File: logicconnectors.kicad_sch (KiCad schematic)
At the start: 28 parts, among them J1 InputConn, J1 USBC Socket, J2 LogicConn2, J3 UART2, J5 HallConn, J6 LogicConn, J7 JTAG, J8 CANConn, U2 USBLC6-2P6, U6 TJA1051T-3

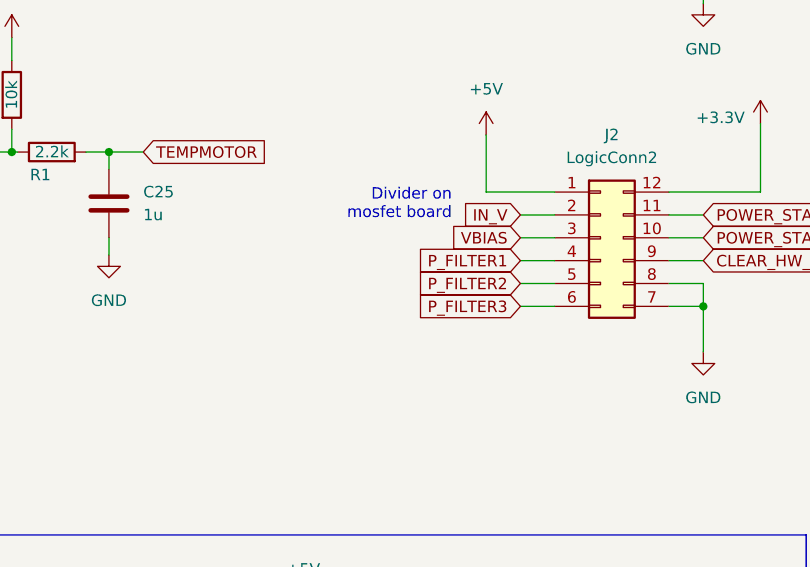
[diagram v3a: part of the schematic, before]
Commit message: initial
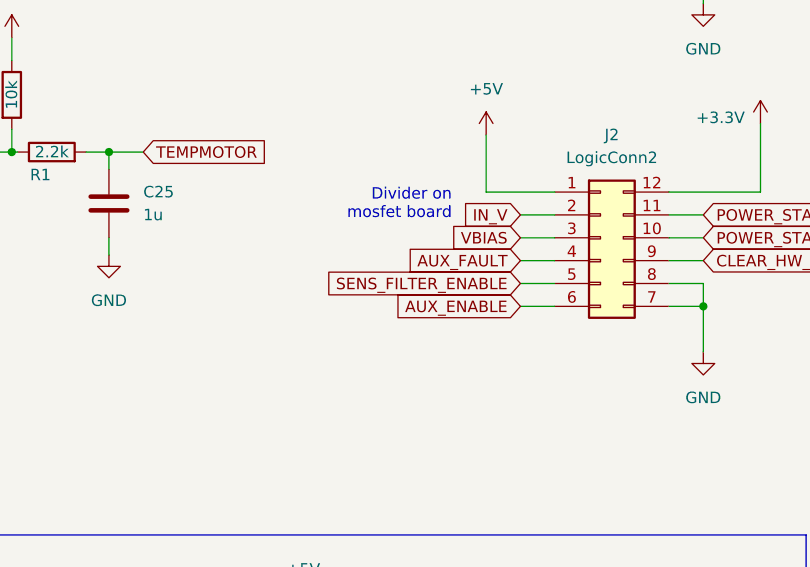
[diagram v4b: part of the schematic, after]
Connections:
- net P_FILTER1 renamed AUX_FAULT
- net P_FILTER2 renamed SENS_FILTER_ENABLE
- net P_FILTER3 renamed AUX_ENABLE
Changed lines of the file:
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@@
+    )
+  )
+  (global_label "SENS_FILTER_ENABLE" (shape input) (at 142.24 101.6 180) (fields_autoplaced)
+    (effects (font (size 1.27 1.27)) (justify right))
+    (property "Intersheetrefs" "${INTERSHEET_REFS}" (at 120.0314 101.6 0)
+      (effects (font (size 1.27 1.27)) (justify right) hide)
     )
   )
@@
     )
   )
+  (global_label "AUX_FAULT" (shape input) (at 142.24 99.06 180) (fields_autoplaced)
+    (effects (font (size 1.27 1.27)) (justify right))
+    (property "Intersheetrefs" "${INTERSHEET_REFS}" (at 129.8888 99.06 0)
+      (effects (font (size 1.27 1.27)) (justify right) hide)
+    )
+  )
   (global_label "MOSTEMP1" (shape input) (at 163.83 52.705 0) (fields_autoplaced)
     (effects (font (size 1.27 1.27)) (justify left))
@@
     )
   )
-  (global_label "P_FILTER3" (shape input) (at 142.24 104.14 180) (fields_autoplaced)
-    (effects (font (size 1.27 1.27)) (justify right))
-    (property "Intersheetrefs" "${INTERSHEET_REFS}" (at 130.4332 104.14 0)
-      (effects (font (size 1.27 1.27)) (justify right) hide)
-    )
-  )
   (global_label "CANTx" (shape input) (at 101.6 160.02 180) (fields_autoplaced)
     (effects (font (size 1.27 1.27)) (justify right))
@@
     )
   )
-  (global_label "P_FILTER1" (shape input) (at 142.24 99.06 180) (fields_autoplaced)
-    (effects (font (size 1.27 1.27)) (justify right))
-    (property "Intersheetrefs" "${INTERSHEET_REFS}" (at 130.4332 99.06 0)
-      (effects (font (size 1.27 1.27)) (justify right) hide)
-    )
-  )
   (global_label "TX_SCL_MOSI" (shape input) (at 38.1 52.07 0) (fields_autoplaced)
     (effects (font (size 1.27 1.27)) (justify left))
@@
     )
   )
-  (global_label "P_FILTER2" (shape input) (at 142.24 101.6 180) (fields_autoplaced)
-    (effects (font (size 1.27 1.27)) (justify right))
-    (property "Intersheetrefs" "${INTERSHEET_REFS}" (at 130.4332 101.6 0)
-      (effects (font (size 1.27 1.27)) (justify right) hide)
-    )
-  )
   (global_label "TX_EXT2" (shape input) (at 41.91 92.075 0) (fields_autoplaced)
     (effects (font (size 1.27 1.27)) (justify left))
@@
     )
   )
+  (global_label "AUX_ENABLE" (shape input) (at 142.24 104.14 180) (fields_autoplaced)
+    (effects (font (size 1.27 1.27)) (justify right))
+    (property "Intersheetrefs" "${INTERSHEET_REFS}" (at 128.377 104.14 0)
+      (effects (font (size 1.27 1.27)) (justify right) hide)
+    )
+  )

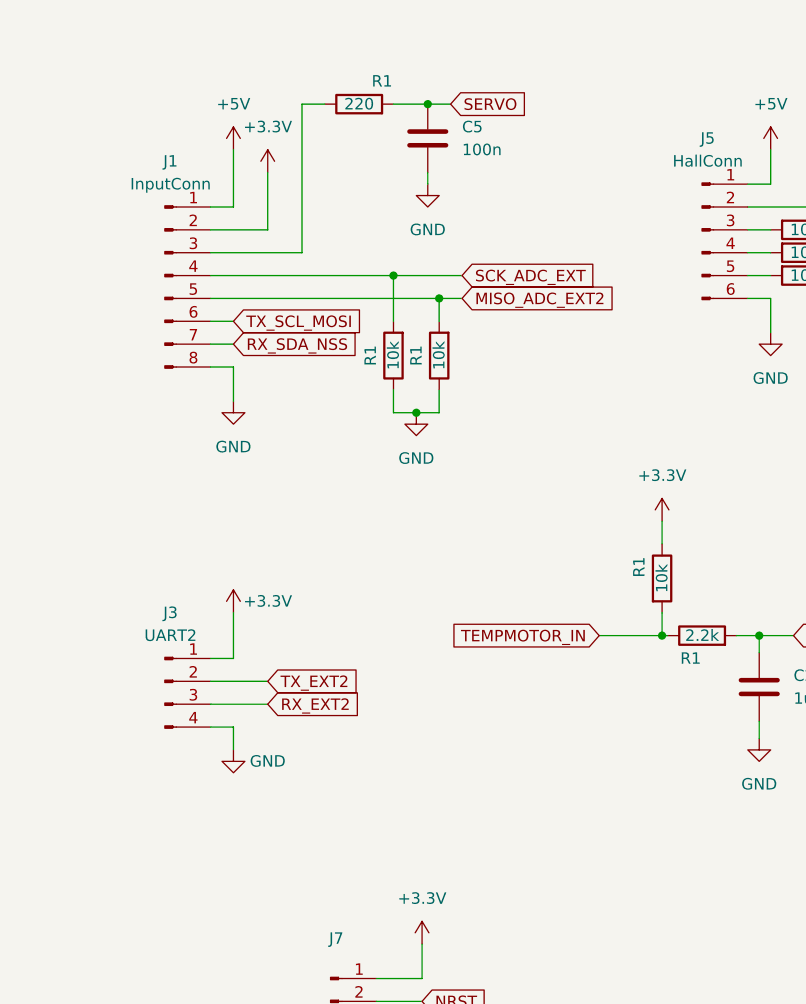
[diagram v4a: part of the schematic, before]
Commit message: jlcpcb
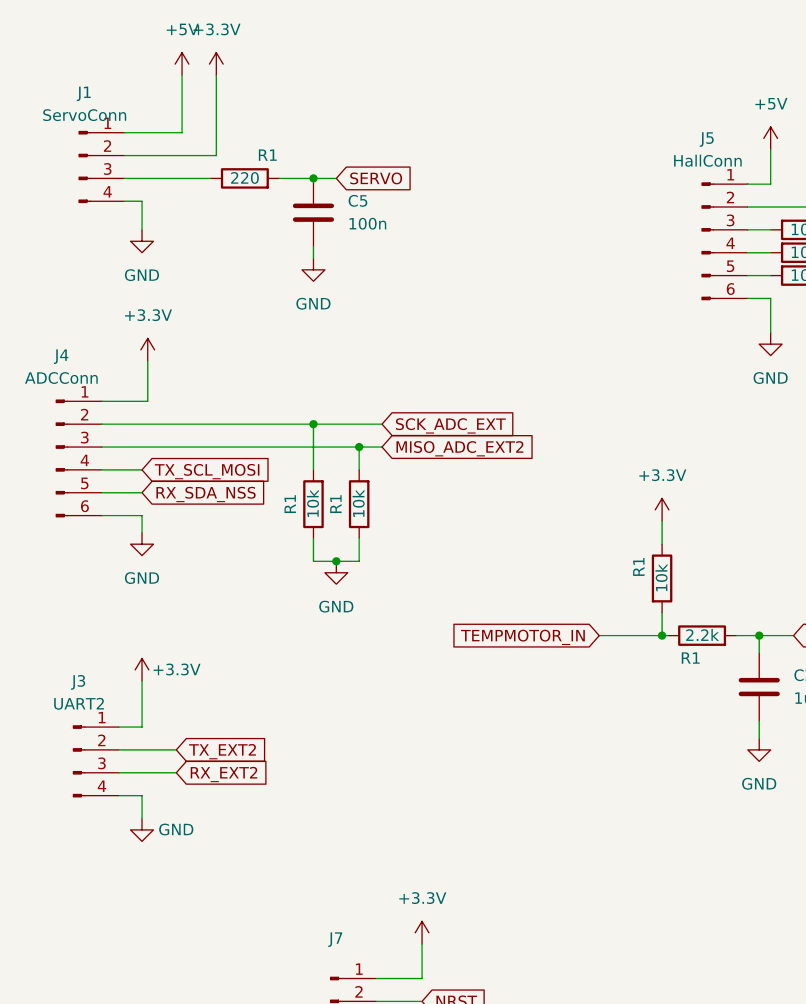
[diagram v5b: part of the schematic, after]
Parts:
- removed J1: InputConn, Connector_PinHeader_2.54mm:PinHeader_1x08_P2.54mm_Horizontal, symbol Connector:Conn_01x08_Pin
- added J1: ServoConn, Connector_JST:JST_EH_S4B-EH_1x04_P2.50mm_Horizontal, symbol Connector:Conn_01x04_Pin
- added J4: ADCConn, Connector_JST:JST_EH_S6B-EH_1x06_P2.50mm_Horizontal, symbol Connector:Conn_01x06_Pin
- C27: MPN (none) -> C377773
- J1: MPN (none) -> C2765186
- J2: MPN (none) -> C225521
- J3, J8: footprint Connector_PinHeader_2.54mm:PinHeader_1x04_P2.54mm_Horizontal -> Connector_JST:JST_EH_S4B-EH_1x04_P2.50mm_Horizontal; MPN (none) -> C265068
- J5: footprint Connector_PinHeader_2.54mm:PinHeader_1x06_P2.54mm_Horizontal -> Connector_JST:JST_EH_S6B-EH_1x06_P2.50mm_Horizontal; MPN (none) -> C495208
- J6: MPN (none) -> C2685199
- J7: MPN (none) -> C124379
- R1: MPN (none) -> C17557
- R1: MPN (none) -> C17408
- R4: MPN (none) -> C17561
- R5: MPN (none) -> C118848
- U2: MPN (none) -> C2827693
- U6: footprint Package_SO:SOIC-8_3.9x4.9mm_P1.27mm -> Package_SO:SOP-8_3.9x4.9mm_P1.27mm; MPN (none) -> C5342108
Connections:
- net +3.3V: now also J1.2 (Pin_2), J4.1 (Pin_1)
- net +5V: now also J1.1 (Pin_1)
- net GND: now also J1.4 (Pin_4), J4.6 (Pin_6)
- net MISO_ADC_EXT2: now also J4.3 (Pin_3)
- net RX_SDA_NSS: now also J4.5 (Pin_5)
- net SCK_ADC_EXT: now also J4.2 (Pin_2)
- net TX_SCL_MOSI: now also J4.4 (Pin_4)
- net at R1.1: now also J1.3 (Pin_3)
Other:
- moved on the sheet: C5, J3, R1

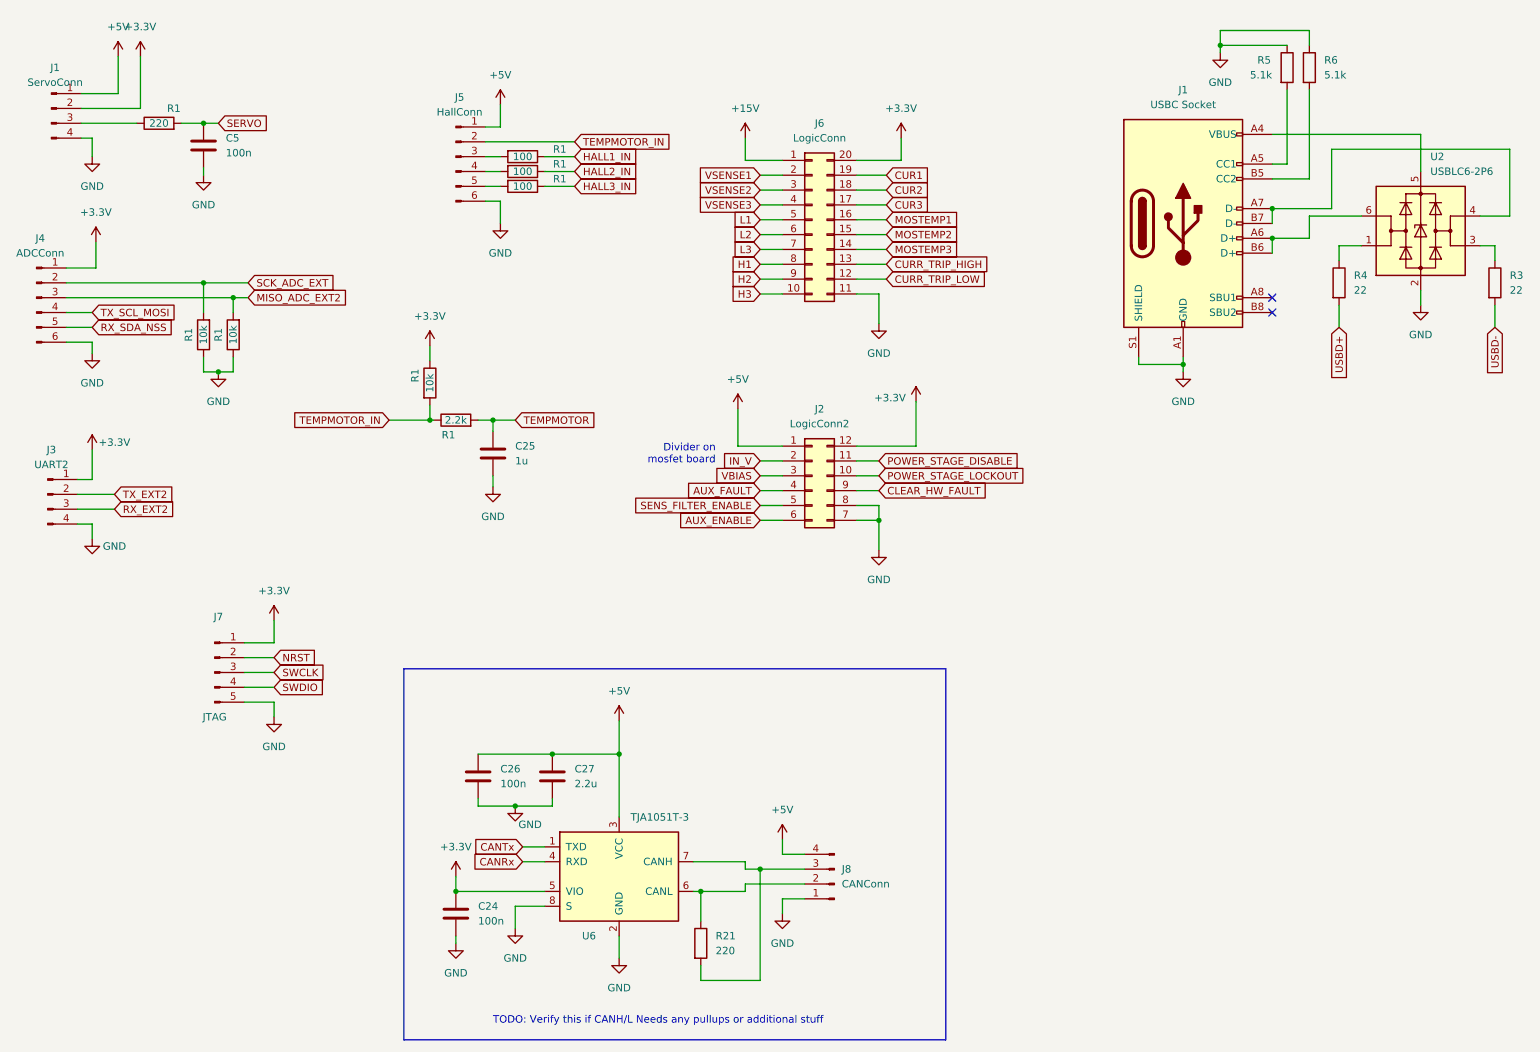
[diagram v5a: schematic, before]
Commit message: routinglogic
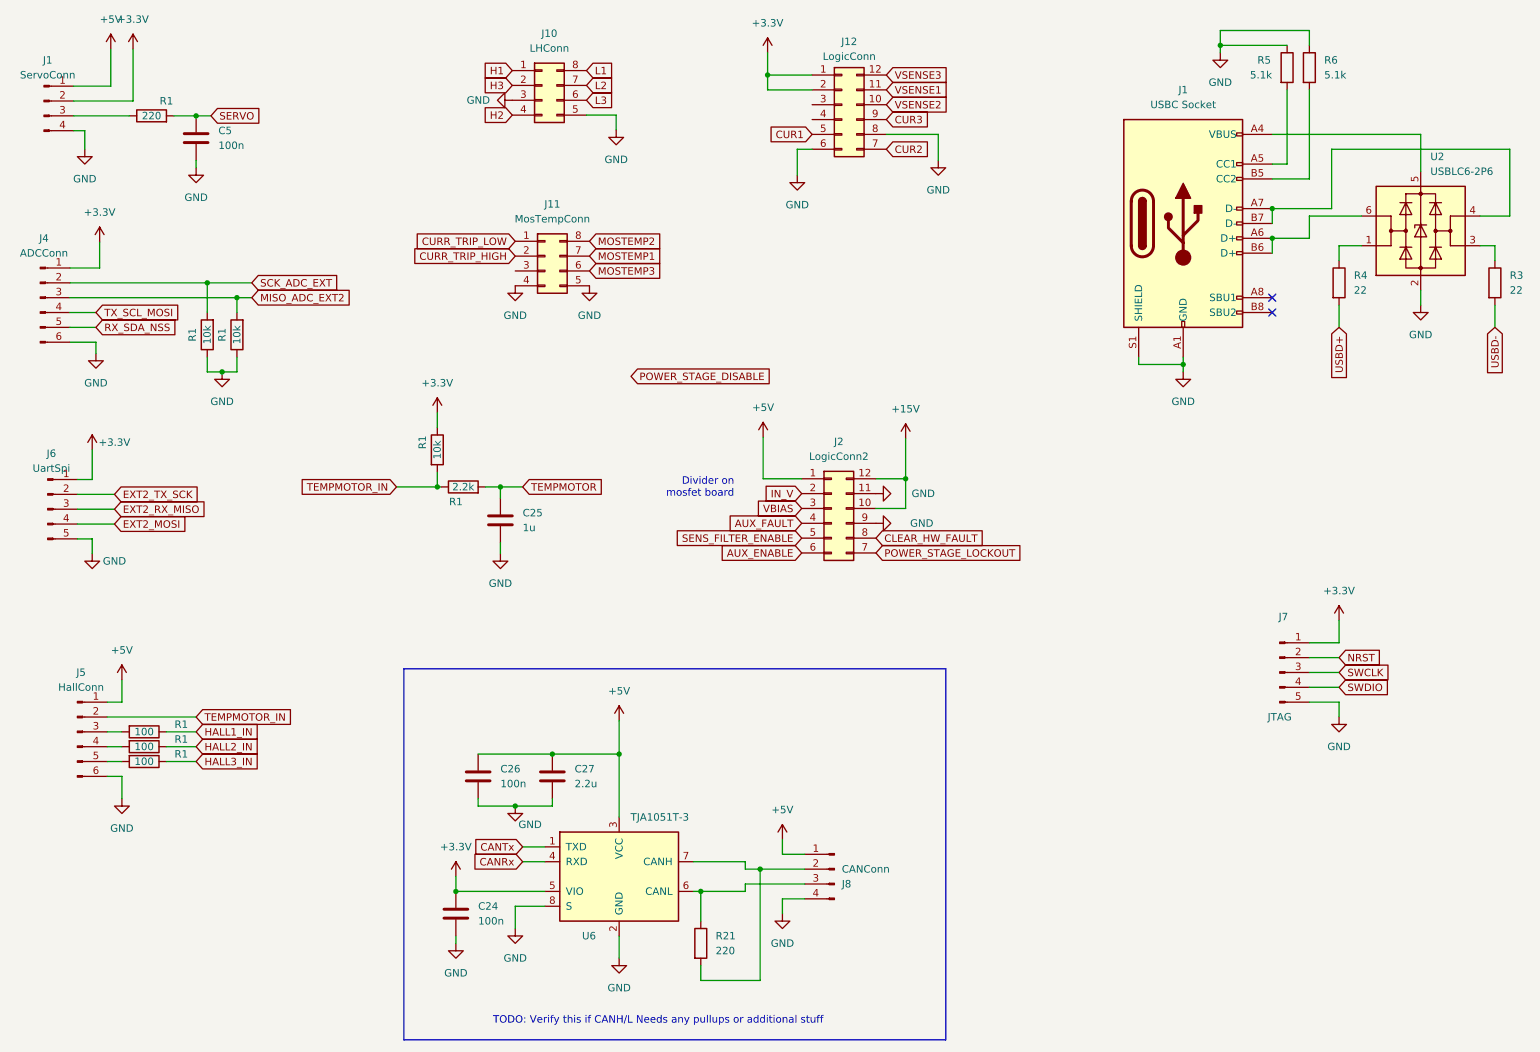
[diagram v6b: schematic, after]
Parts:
- removed J3: UART2, Connector_JST:JST_EH_S4B-EH_1x04_P2.50mm_Horizontal, symbol Connector:Conn_01x04_Pin
- removed J6: LogicConn, Connector_PinHeader_2.54mm:PinHeader_2x10_P2.54mm_Vertical, symbol Connector_Generic:Conn_02x10_Counter_Clockwise
- added J10: LHConn, Connector_PinHeader_2.54mm:PinHeader_2x04_P2.54mm_Vertical, symbol Connector_Generic:Conn_02x04_Counter_Clockwise
- added J11: MosTempConn, Connector_PinHeader_2.54mm:PinHeader_2x04_P2.54mm_Vertical, symbol Connector_Generic:Conn_02x04_Counter_Clockwise
- added J12: LogicConn, Connector_PinHeader_2.54mm:PinHeader_2x06_P2.54mm_Vertical, symbol Connector_Generic:Conn_02x06_Counter_Clockwise
- added J6: UartSpi, Connector_JST:JST_EH_S5B-EH_1x05_P2.50mm_Horizontal, symbol Connector:Conn_01x05_Pin
- J1: JLCPosOffset (none) -> 0,1.27
- J1, J8: JLCPosOffset (none) -> 3.75,0
- J4, J5: JLCPosOffset (none) -> 6.25,0
- J7: JLCPosOffset (none) -> 5.08,0; JLCRotOffset (none) -> -90
- U2, U6: JLCRotOffset (none) -> -90
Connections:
- net +15V: now also J2.10 (Pin_10), J2.12 (Pin_12)
- net +3.3V: now also J12.1 (Pin_1), J12.2 (Pin_2), J6.1 (Pin_1); no longer J2.12 (Pin_12)
- net +5V: now also J8.1 (Pin_1); no longer J8.4 (Pin_4)
- net CLEAR_HW_FAULT: now also J2.8 (Pin_8); no longer J2.9 (Pin_9)
- net CUR1: now also J12.5 (Pin_5)
- net CUR2: now also J12.7 (Pin_7)
- net CUR3: now also J12.9 (Pin_9)
- net CURR_TRIP_HIGH: now also J11.2 (Pin_2)
- net CURR_TRIP_LOW: now also J11.1 (Pin_1)
- net GND: now also J2.11 (Pin_11), J2.9 (Pin_9), J8.4 (Pin_4), J10.3 (Pin_3), J10.5 (Pin_5), J11.4 (Pin_4), J11.5 (Pin_5), J12.6 (Pin_6), J12.8 (Pin_8), J6.5 (Pin_5); no longer J2.7 (Pin_7), J2.8 (Pin_8), J8.1 (Pin_1)
- net H1: now also J10.1 (Pin_1)
- net H2: now also J10.4 (Pin_4)
- net H3: now also J10.2 (Pin_2)
- net L1: now also J10.8 (Pin_8)
- net L2: now also J10.7 (Pin_7)
- net L3: now also J10.6 (Pin_6)
- net MOSTEMP1: now also J11.7 (Pin_7)
- net MOSTEMP2: now also J11.8 (Pin_8)
- net MOSTEMP3: now also J11.6 (Pin_6)
- net POWER_STAGE_DISABLE: no longer J2.11 (Pin_11)
- net POWER_STAGE_LOCKOUT: now also J2.7 (Pin_7); no longer J2.10 (Pin_10)
- net VSENSE1: now also J12.11 (Pin_11)
- net VSENSE2: now also J12.10 (Pin_10)
- net VSENSE3: now also J12.12 (Pin_12)
- net at R21.1, U6.6 (CANL): now also J8.3 (Pin_3); no longer J8.2 (Pin_2)
- net at R21.2, U6.7 (CANH): now also J8.2 (Pin_2); no longer J8.3 (Pin_3)
- new net EXT2_MOSI: J6.4 (Pin_4)
- new net EXT2_RX_MISO: J6.3 (Pin_3)
- new net EXT2_TX_SCK: J6.2 (Pin_2)
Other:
- moved on the sheet: C25, C5, J1, J2, J4, J5, J7, J8, R1
